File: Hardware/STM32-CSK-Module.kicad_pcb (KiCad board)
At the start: 2 copper layers, 32 parts, among them J1 Conn_Cortex-JTAG-10, U1 STM32F417VGT, X1 8MHz, X2 32.768kHz

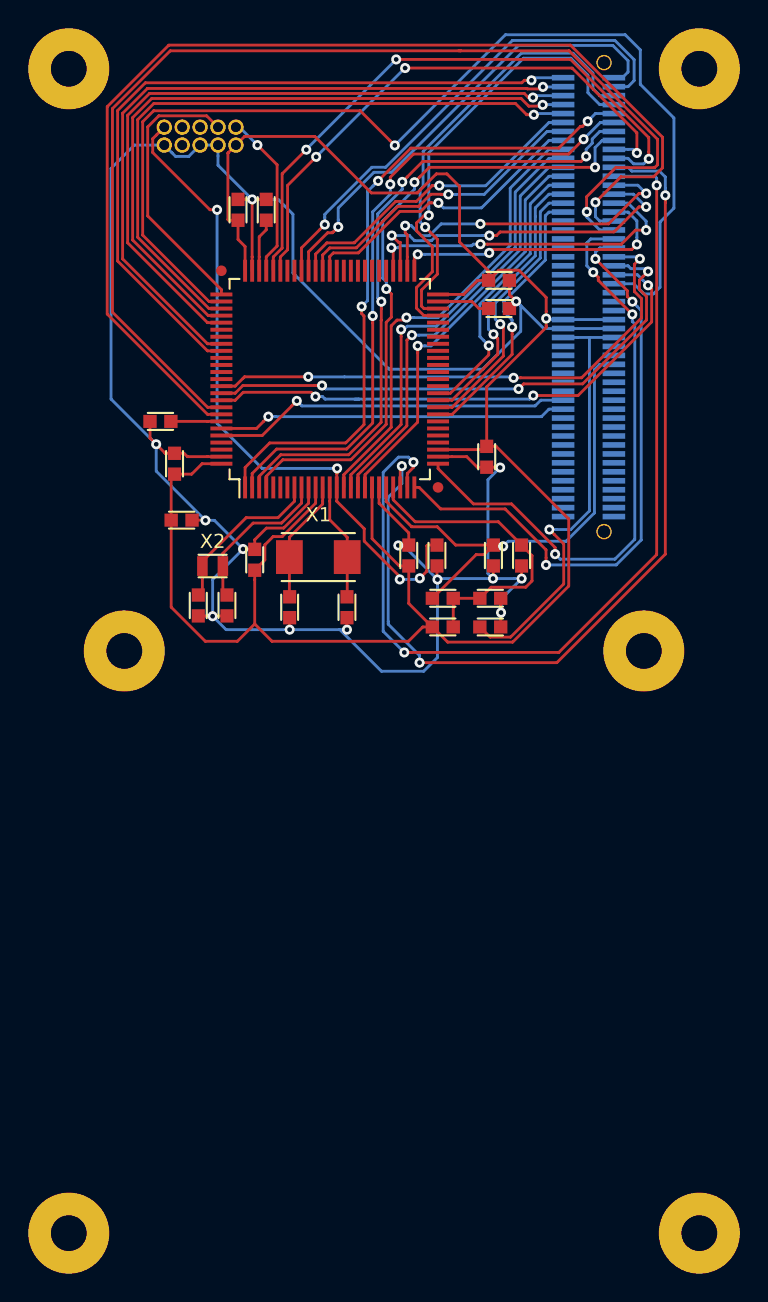
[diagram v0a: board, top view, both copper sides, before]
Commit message: Done. Moderately clean.
All used pins routed.
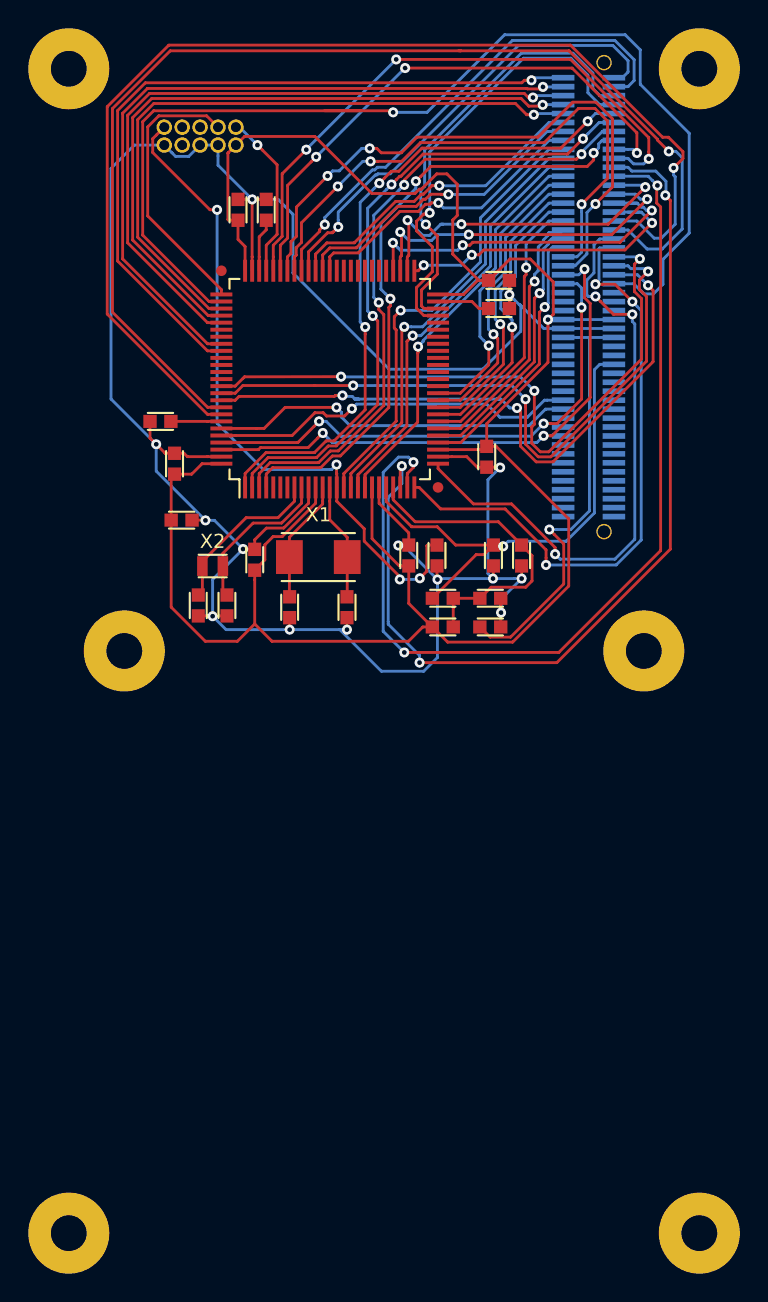
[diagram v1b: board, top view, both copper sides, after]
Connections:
- H1 pad 33: Net-(H1-Pad33) -> /IO31
- H1 pad 35: Net-(H1-Pad35) -> /IO30
- H1 pad 37: Net-(H1-Pad37) -> /IO29
- H1 pad 39: Net-(H1-Pad39) -> /IO28
- H1 pad 41: Net-(H1-Pad41) -> /IO27
- H1 pad 43: Net-(H1-Pad43) -> /IO26
- H1 pad 45: Net-(H1-Pad45) -> /IO25
- H1 pad 47: Net-(H1-Pad47) -> /IO24
- U1 pad 29: Net-(U1-Pad29) -> /IO28
- U1 pad 30: Net-(U1-Pad30) -> /IO29
- U1 pad 31: Net-(U1-Pad31) -> /IO30
- U1 pad 32: Net-(U1-Pad32) -> /IO31
- U1 pad 68: Net-(U1-Pad68) -> /IO27
- U1 pad 69: Net-(U1-Pad69) -> /IO26
- U1 pad 97: Net-(U1-Pad97) -> /IO24
- U1 pad 98: Net-(U1-Pad98) -> /IO25
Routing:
- net /IO26: track 0.00 -> 43.4 mm, vias 0 -> 3
- net /IO27: track 0.00 -> 40.5 mm, vias 0 -> 3
- net /IO25: track 0.00 -> 39.2 mm, vias 0 -> 3
- net /IO24: track 0.00 -> 37.0 mm, vias 0 -> 3
- net /IO28: track 0.00 -> 19.5 mm, vias 0 -> 1
- net /IO30: track 0.00 -> 19.4 mm, vias 0 -> 1
- net /IO31: track 0.00 -> 19.4 mm, vias 0 -> 1
- net /IO29: track 0.00 -> 19.0 mm, vias 0 -> 1
- net /SPI1_SCK: track 38.3 -> 46.8 mm
- net /SPI1_MISO: track 39.0 -> 46.5 mm
- net /SPI1_MOSI: track 38.9 -> 46.2 mm
- net +3V3: track 148.6 -> 151.1 mm
- net /USART1_RX: track 80.0 -> 82.2 mm
- net /USART1_TX: track 79.7 -> 81.4 mm
- net /~SPI1_SS: track 77.9 -> 79.4 mm
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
